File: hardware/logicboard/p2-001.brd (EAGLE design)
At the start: 72 x 72 mm, 51 parts, among them IC1 4066N, IC2 LTC485N, IC3 74LS07N, J1 LED, J2 RLY, J3 PWR, J4 DC9V, J5 Display, K1 G5V1, T1 2SC1815, U1 DS18B20

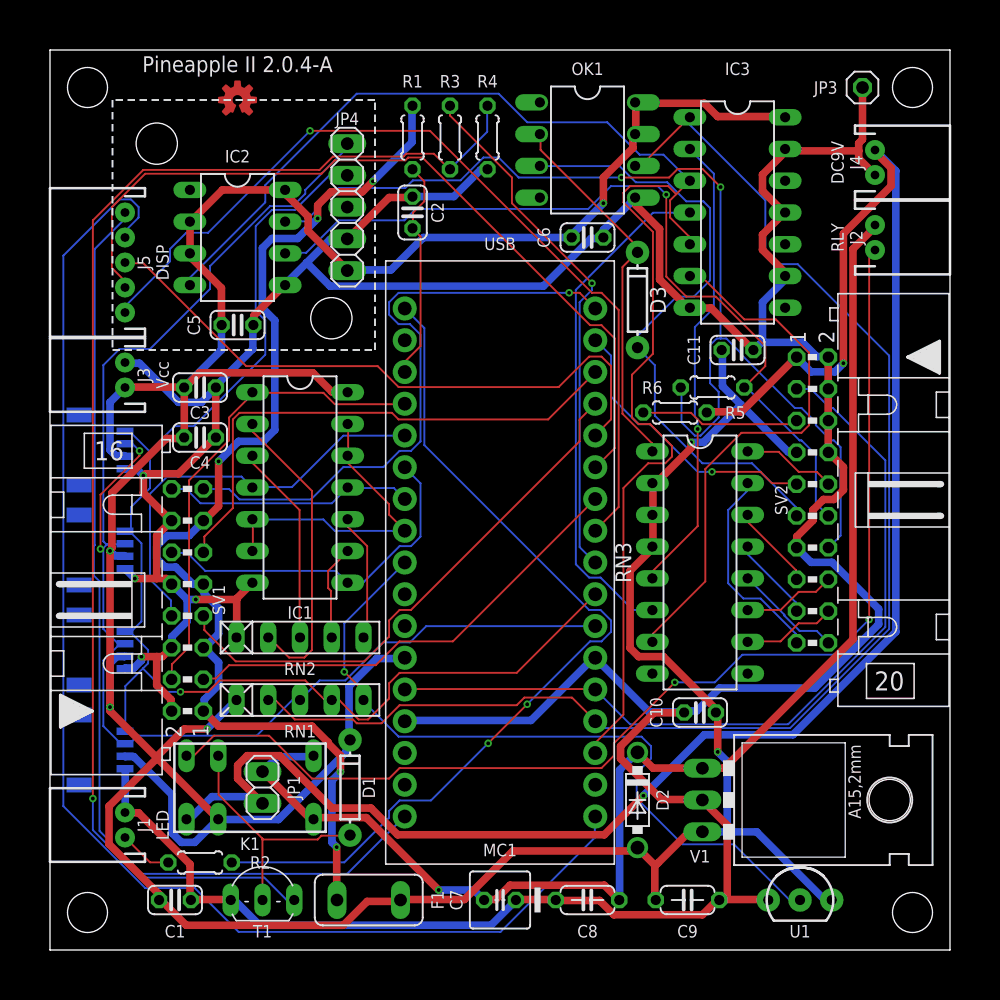
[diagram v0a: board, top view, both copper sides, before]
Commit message: To be renumbered.
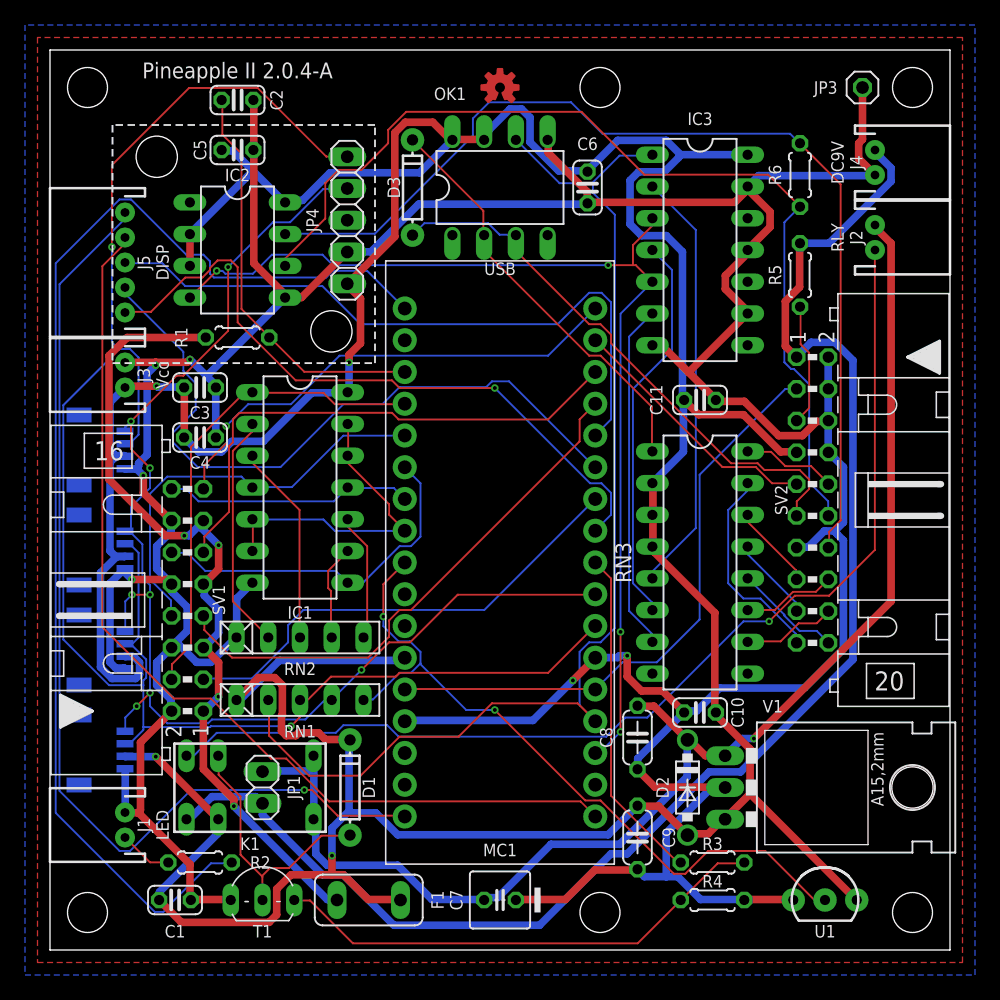
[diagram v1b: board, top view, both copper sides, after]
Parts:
- moved R4 63.6 mm to (53.0, 4.00), turned to 180 degrees
- moved R3 61.7 mm to (53.0, 7.00), turned to 180 degrees
- moved R1 21.3 mm to (15.0, 49.0), turned to 180 degrees
- moved LOGO1 21.0 mm to (36.0, 69.0)
- moved D3 20.1 mm to (29.0, 61.0)
- moved R6 18.4 mm to (60.0, 62.0), turned to 90 degrees
- moved C2 16.6 mm to (15.0, 68.0), turned to 0 degrees
- moved R5 14.9 mm to (60.0, 54.0), turned to 90 degrees
- moved C5 14.0 mm to (15.0, 64.0)
- moved C8 13.6 mm to (47.0, 17.0), turned to 270 degrees
- moved OK1 7.62 mm to (36.0, 61.0), turned to 0 degrees
- moved C9 6.40 mm to (47.0, 9.00), turned to 270 degrees
- moved C11 5.00 mm to (52.0, 44.0)
- moved IC3 4.24 mm to (52.0, 56.0)
- moved D2 4.12 mm to (51.0, 13.0)
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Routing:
- net RLYDRV: track 104.8 -> 40.1 mm, vias 1 -> 0
- net TX: track 113.2 -> 83.7 mm, vias 0 -> 4
- net MOSI: track 106.6 -> 77.7 mm
- net LED0: track 71.5 -> 97.7 mm, vias 2 -> 0
- net +9V: track 145.2 -> 119.6 mm, vias 2 -> 0
- net SDA: track 115.5 -> 140.7 mm
- net +5V: track 91.8 -> 66.6 mm, vias 5 -> 4
- net VCC: track 327.8 -> 348.5 mm, vias 6 -> 4
- net RST: track 65.7 -> 48.1 mm
- net RX: track 109.9 -> 92.7 mm
- net DISP1: track 70.7 -> 54.6 mm
- net MO2: track 43.2 -> 27.8 mm
- net RLY: track 42.2 -> 27.0 mm, vias 1 -> 0
- net AREF: track 17.8 -> 32.6 mm
- net MTX+: track 67.1 -> 78.9 mm, vias 1 -> 0
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- added copper zone on layer 1, net GND
- added copper zone on layer 16, net GND
